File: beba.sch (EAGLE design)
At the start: 37 parts, among them IC1 LT1302SO08, IC2 MCP73871-2AAI/ML

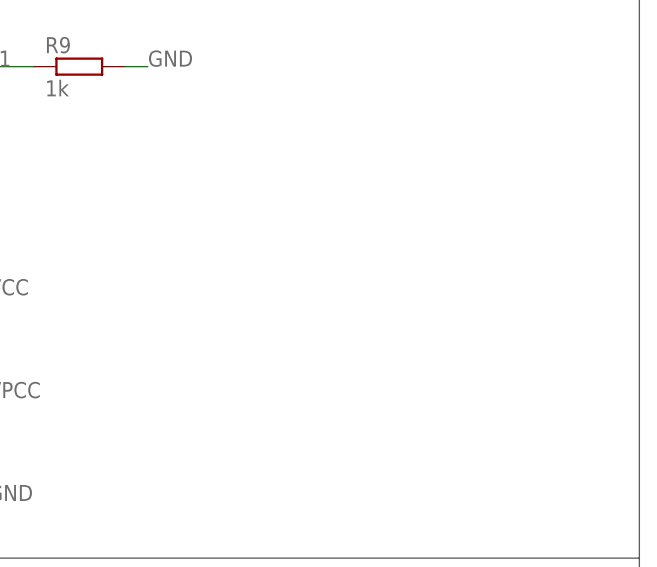
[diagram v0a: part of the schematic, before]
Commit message: - further minor corrections
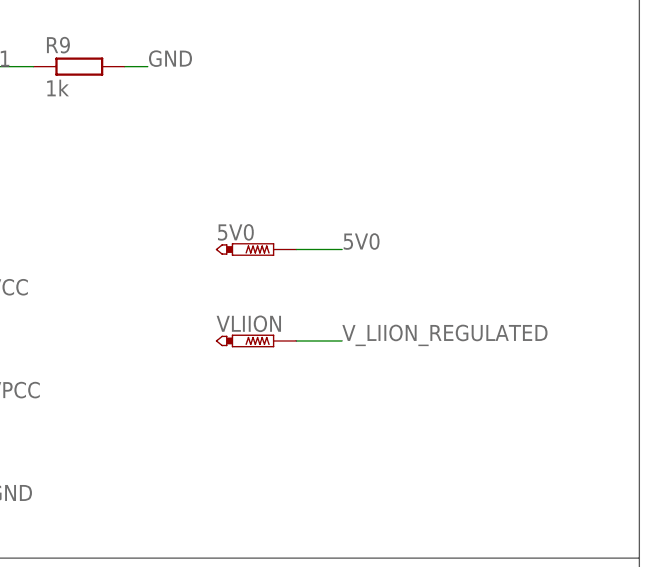
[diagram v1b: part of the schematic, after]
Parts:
- added 5V0, VLIION: PTR1B2,54, testpad:PTR1B2,54
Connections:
- net 5V0: now also 5V0.TP
- net V_LIION_REGULATED: now also VLIION.TP
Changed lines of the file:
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@@
 <grid distance="0.1" unitdist="inch" unit="inch" style="lines" multiple="1" display="yes" altdistance="0.01" altunitdist="inch" altunit="inch"/>
 <layers>
-<layer number="1" name="Top" color="4" fill="1" visible="no" active="no"/>
-<layer number="2" name="Route2" color="1" fill="3" visible="no" active="no"/>
-<layer number="3" name="Route3" color="4" fill="3" visible="no" active="no"/>
-<layer number="4" name="Route4" color="1" fill="4" visible="no" active="no"/>
-<layer number="5" name="Route5" color="4" fill="4" visible="no" active="no"/>
-<layer number="6" name="Route6" color="1" fill="8" visible="no" active="no"/>
-<layer number="7" name="Route7" color="4" fill="8" visible="no" active="no"/>
-<layer number="8" name="Route8" color="1" fill="2" visible="no" active="no"/>
-<layer number="9" name="Route9" color="4" fill="2" visible="no" active="no"/>
-<layer number="10" name="Route10" color="1" fill="7" visible="no" active="no"/>
-<layer number="11" name="Route11" color="4" fill="7" visible="no" active="no"/>
-<layer number="12" name="Route12" color="1" fill="5" visible="no" active="no"/>
-<layer number="13" name="Route13" color="4" fill="5" visible="no" active="no"/>
-<layer number="14" name="Route14" color="1" fill="6" visible="no" active="no"/>
-<layer number="15" name="Route15" color="4" fill="6" visible="no" active="no"/>
-<layer number="16" name="Bottom" color="1" fill="1" visible="no" active="no"/>
-<layer number="17" name="Pads" color="2" fill="1" visible="no" active="no"/>
-<layer number="18" name="Vias" color="2" fill="1" visible="no" active="no"/>
-<layer number="19" name="Unrouted" color="6" fill="1" visible="no" active="no"/>
-<layer number="20" name="Dimension" color="15" fill="1" visible="no" active="no"/>
-<layer number="21" name="tPlace" color="7" fill="1" visible="no" active="no"/>
-<layer number="22" name="bPlace" color="7" fill="1" visible="no" active="no"/>
-<layer number="23" name="tOrigins" color="15" fill="1" visible="no" active="no"/>
-<layer number="24" name="bOrigins" color="15" fill="1" visible="no" active="no"/>
-<layer number="25" name="tNames" color="7" fill="1" visible="no" active="no"/>
-<layer number="26" name="bNames" color="7" fill="1" visible="no" active="no"/>
-<layer number="27" name="tValues" color="7" fill="1" visible="no" active="no"/>
-<layer number="28" name="bValues" color="7" fill="1" visible="no" active="no"/>
+<layer number="1" name="Top" color="4" fill="1" visible="yes" active="no"/>
+<layer number="2" name="Route2" color="1" fill="3" visible="yes" active="no"/>
+<layer number="3" name="Route3" color="4" fill="3" visible="yes" active="no"/>
+<layer number="4" name="Route4" color="1" fill="4" visible="yes" active="no"/>
+<layer number="5" name="Route5" color="4" fill="4" visible="yes" active="no"/>
+<layer number="6" name="Route6" color="1" fill="8" visible="yes" active="no"/>
+<layer number="7" name="Route7" color="4" fill="8" visible="yes" active="no"/>
+<layer number="8" name="Route8" color="1" fill="2" visible="yes" active="no"/>
+<layer number="9" name="Route9" color="4" fill="2" visible="yes" active="no"/>
+<layer number="10" name="Route10" color="1" fill="7" visible="yes" active="no"/>
+<layer number="11" name="Route11" color="4" fill="7" visible="yes" active="no"/>
+<layer number="12" name="Route12" color="1" fill="5" visible="yes" active="no"/>
+<layer number="13" name="Route13" color="4" fill="5" visible="yes" active="no"/>
+<layer number="14" name="Route14" color="1" fill="6" visible="yes" active="no"/>
+<layer number="15" name="Route15" color="4" fill="6" visible="yes" active="no"/>
+<layer number="16" name="Bottom" color="1" fill="1" visible="yes" active="no"/>
+<layer number="17" name="Pads" color="2" fill="1" visible="yes" active="no"/>
+<layer number="18" name="Vias" color="2" fill="1" visible="yes" active="no"/>
+<layer number="19" name="Unrouted" color="6" fill="1" visible="yes" active="no"/>
+<layer number="20" name="Dimension" color="15" fill="1" visible="yes" active="no"/>
+<layer number="21" name="tPlace" color="7" fill="1" visible="yes" active="no"/>
+<layer number="22" name="bPlace" color="7" fill="1" visible="yes" active="no"/>
+<layer number="23" name="tOrigins" color="15" fill="1" visible="yes" active="no"/>
+<layer number="24" name="bOrigins" color="15" fill="1" visible="yes" active="no"/>
+<layer number="25" name="tNames" color="7" fill="1" visible="yes" active="no"/>
+<layer number="26" name="bNames" color="7" fill="1" visible="yes" active="no"/>
+<layer number="27" name="tValues" color="7" fill="1" visible="yes" active="no"/>
+<layer number="28" name="bValues" color="7" fill="1" visible="yes" active="no"/>
 <layer number="29" name="tStop" color="7" fill="3" visible="no" active="no"/>
 <layer number="30" name="bStop" color="7" fill="6" visible="no" active="no"/>
@@
 <layer number="35" name="tGlue" color="7" fill="4" visible="no" active="no"/>
 <layer number="36" name="bGlue" color="7" fill="5" visible="no" active="no"/>
-<layer number="37" name="tTest" color="7" fill="1" visible="no" active="no"/>
-<layer number="38" name="bTest" color="7" fill="1" visible="no" active="no"/>
+<layer number="37" name="tTest" color="7" fill="1" visible="yes" active="no"/>
+<layer number="38" name="bTest" color="7" fill="1" visible="yes" active="no"/>
 <layer number="39" name="tKeepout" color="4" fill="11" visible="no" active="no"/>
 <layer number="40" name="bKeepout" color="1" fill="11" visible="no" active="no"/>
@@
 <layer number="44" name="Drills" color="7" fill="1" visible="no" active="no"/>
 <layer number="45" name="Holes" color="7" fill="1" visible="no" active="no"/>
-<layer number="46" name="Milling" color="3" fill="1" visible="no" active="no"/>
-<layer number="47" name="Measures" color="7" fill="1" visible="no" active="no"/>
-<layer number="48" name="Document" color="7" fill="1" visible="no" active="no"/>
-<layer number="49" name="Reference" color="7" fill="1" visible="no" active="no"/>
-<layer number="50" name="dxf" color="7" fill="1" visible="no" active="no"/>
-<layer number="51" name="tDocu" color="7" fill="1" visible="no" active="no"/>
-<layer number="52" name="bDocu" color="7" fill="1" visible="no" active="no"/>
-<layer number="53" name="tGND_GNDA" color="7" fill="9" visible="no" active="no"/>
-<layer number="54" name="bGND_GNDA" color="1" fill="9" visible="no" active="no"/>
-<layer number="56" name="wert" color="7" fill="1" visible="no" active="no"/>
-<layer number="57" name="tCAD" color="7" fill="1" visible="no" active="no"/>
-<layer number="59" name="tCarbon" color="7" fill="1" visible="no" active="no"/>
-<layer number="60" name="bCarbon" color="7" fill="1" visible="no" active="no"/>
+<layer number="46" name="Milling" color="3" fill="1" visible="yes" active="no"/>
+<layer number="47" name="Measures" color="7" fill="1" visible="yes" active="no"/>
+<layer number="48" name="Document" color="7" fill="1" visible="yes" active="no"/>
+<layer number="49" name="Reference" color="7" fill="1" visible="yes" active="no"/>
+<layer number="50" name="dxf" color="7" fill="1" visible="yes" active="no"/>
+<layer number="51" name="tDocu" color="7" fill="1" visible="yes" active="no"/>
+<layer number="52" name="bDocu" color="7" fill="1" visible="yes" active="no"/>
+<layer number="53" name="tGND_GNDA" color="7" fill="9" visible="yes" active="no"/>
+<layer number="54" name="bGND_GNDA" color="1" fill="9" visible="yes" active="no"/>
+<layer number="56" name="wert" color="7" fill="1" visible="yes" active="no"/>
+<layer number="57" name="tCAD" color="7" fill="1" visible="yes" active="no"/>
+<layer number="59" name="tCarbon" color="7" fill="1" visible="yes" active="no"/>
+<layer number="60" name="bCarbon" color="7" fill="1" visible="yes" active="no"/>
 <layer number="90" name="Modules" color="5" fill="1" visible="yes" active="yes"/>
 <layer number="91" name="Nets" color="2" fill="1" visible="yes" active="yes"/>
@@
 <part name="C9" library="rcl" deviceset="CPOL-EU" device="E2,5-6E" value="4700μF / 10V"/>
 <part name="L" library="DE1205-18 Power Inductor" deviceset="DE1205-18" device=""/>
+<part name="5V0" library="testpad" deviceset="PTR1" device="B2,54"/>
+<part name="VLIION" library="testpad" deviceset="PTR1" device="B2,54"/>
 </parts>
 <sheets>
@@
 <instance part="C9" gate="G$1" x="319.532" y="151.13" rot="R180"/>
 <instance part="L" gate="G$1" x="73.66" y="114.3"/>
+<instance part="5V0" gate="G$1" x="322.58" y="99.06" rot="R270"/>
+<instance part="VLIION" gate="G$1" x="322.58" y="88.9" rot="R270"/>
 </instances>
 <busses>
@@
 <wire x1="135.89" y1="21.59" x2="139.7" y2="21.59" width="0.1524" layer="91"/>
 <label x="139.7" y="21.59" size="1.778" layer="95"/>
+</segment>
+<segment>
+<pinref part="VLIION" gate="G$1" pin="TP"/>
+<wire x1="325.12" y1="88.9" x2="330.2" y2="88.9" width="0.1524" layer="91"/>
+<label x="330.2" y="88.9" size="1.778" layer="95"/>
 </segment>
 </net>
@@
 <label x="327.66" y="148.59" size="1.778" layer="95"/>
 </segment>
+<segment>
+<pinref part="5V0" gate="G$1" pin="TP"/>
+<wire x1="325.12" y1="99.06" x2="330.2" y2="99.06" width="0.1524" layer="91"/>
+<label x="330.2" y="99.06" size="1.778" layer="95"/>
+</segment>
 </net>
 <net name="STAT2" class="2">
@@
 </segment>
 </net>
-<net name="N$4" class="0">
+<net name="N$4" class="1">
 <segment>
 <pinref part="D2" gate="1" pin="A"/>
